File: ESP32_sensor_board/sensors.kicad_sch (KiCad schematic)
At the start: 18 parts, among them Q1 TEMT6000X01, U2 BME280, U7 MAX4466EXK

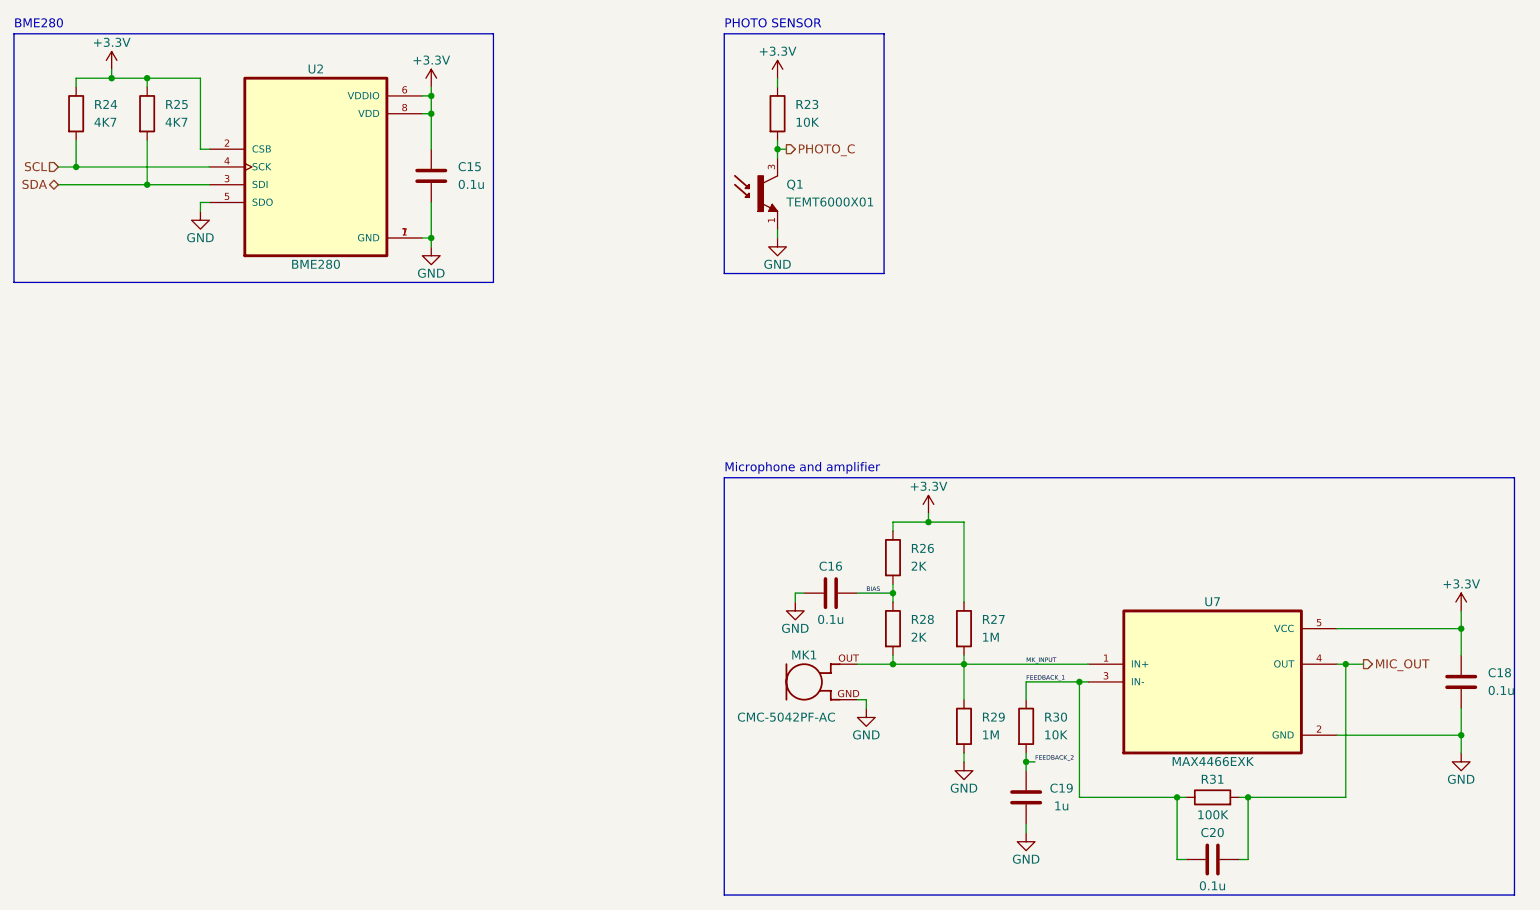
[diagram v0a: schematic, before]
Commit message: Layout design section 2 completed
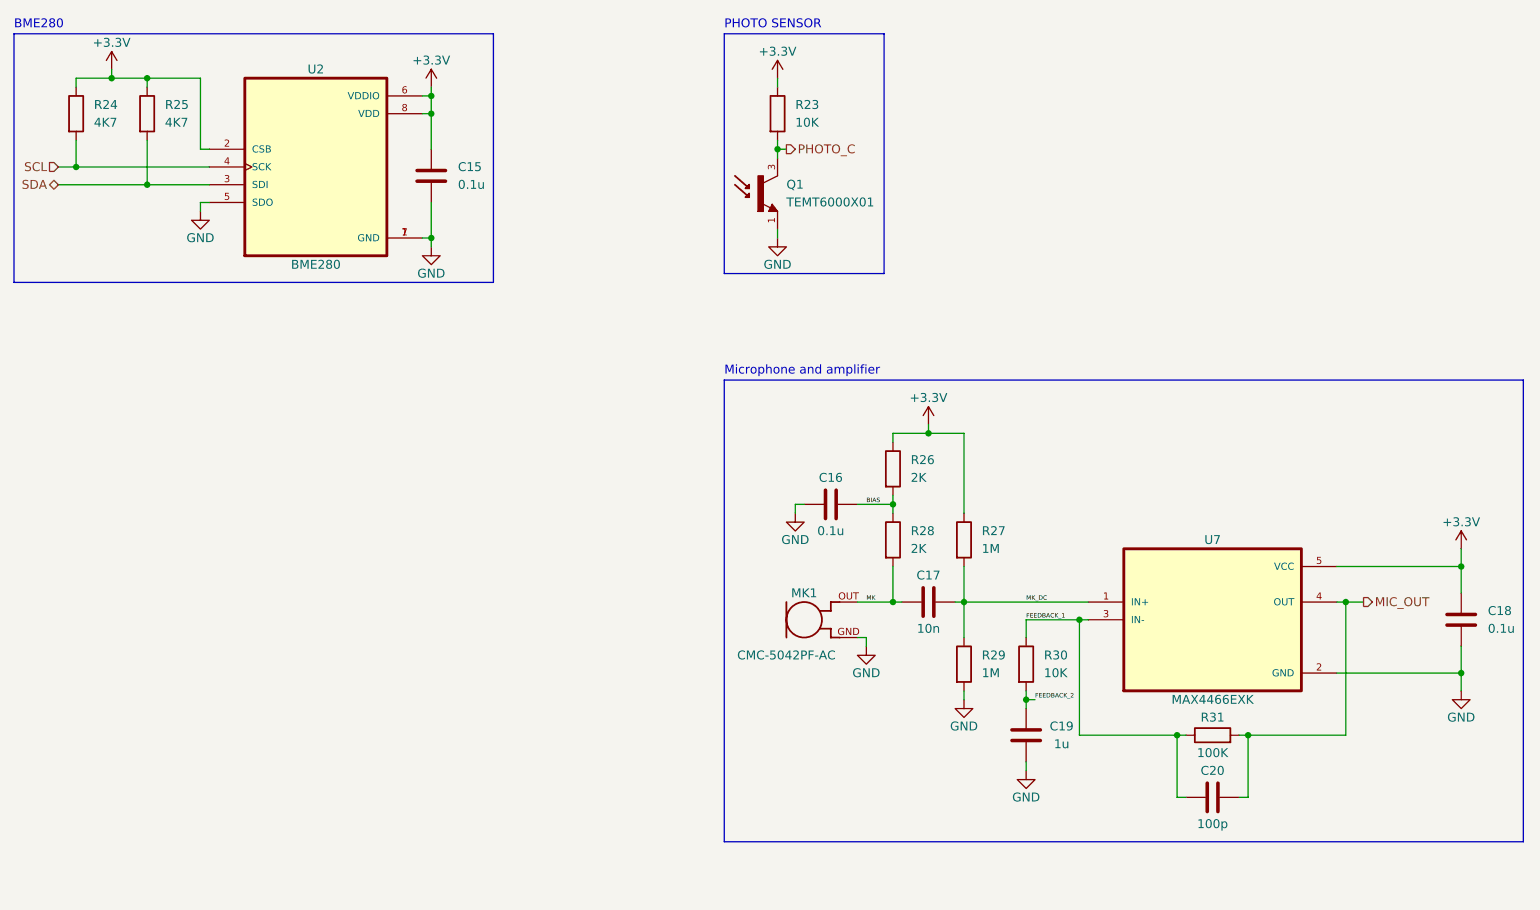
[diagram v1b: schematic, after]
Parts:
- added C17: 10n, Capacitor_SMD:C_0805_2012Metric, symbol Device:C
- C20: value 0.1u -> 100p
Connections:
- net MK_INPUT renamed MK_DC
- net MK_DC: now also C17.2; no longer MK1.OUT, R28.2
- new net MK: C17.1, MK1.OUT, R28.2
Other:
- moved on the sheet: C16, C18, C19, C20, MK1, R26, R27, R28, R29, R30, R31, U7
